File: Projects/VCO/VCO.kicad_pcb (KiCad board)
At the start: 2 copper layers, 13.2 x 38.4 mm, 33 parts, among them J1 Conn_01x02, J3 Conn_01x02, Q1 BFR193, Q2 BFR193

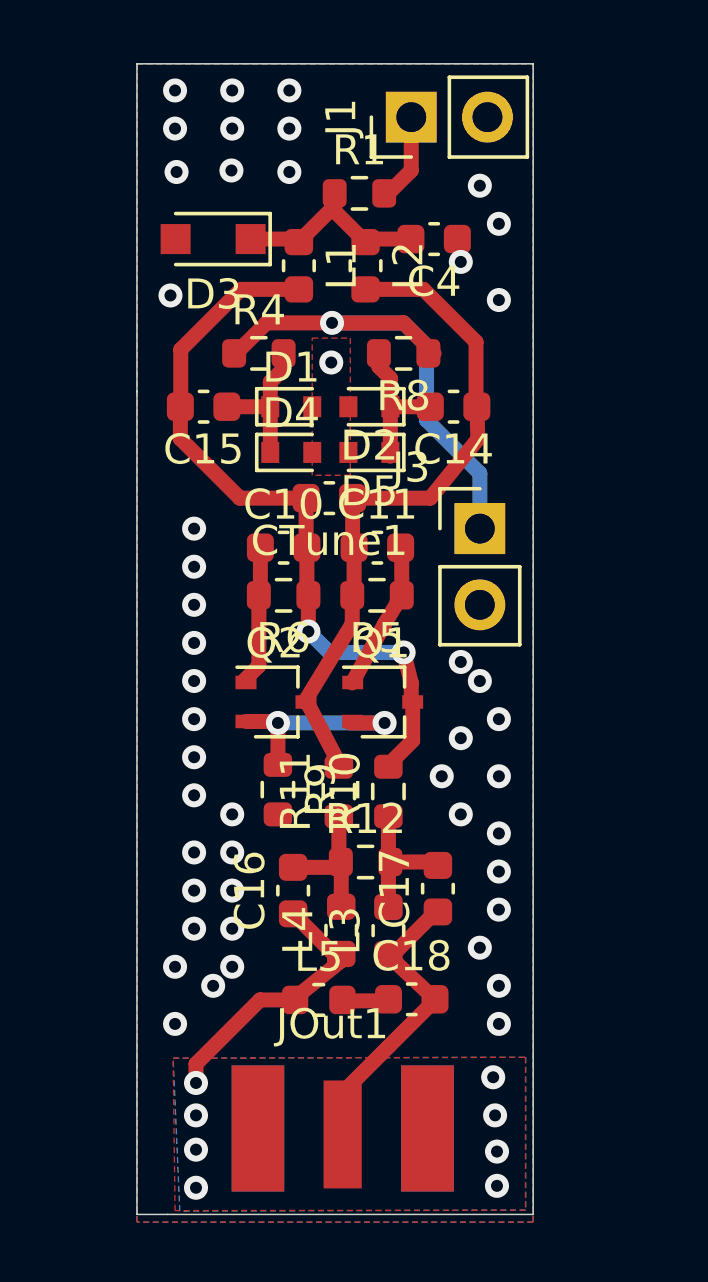
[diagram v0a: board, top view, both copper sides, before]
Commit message: last update
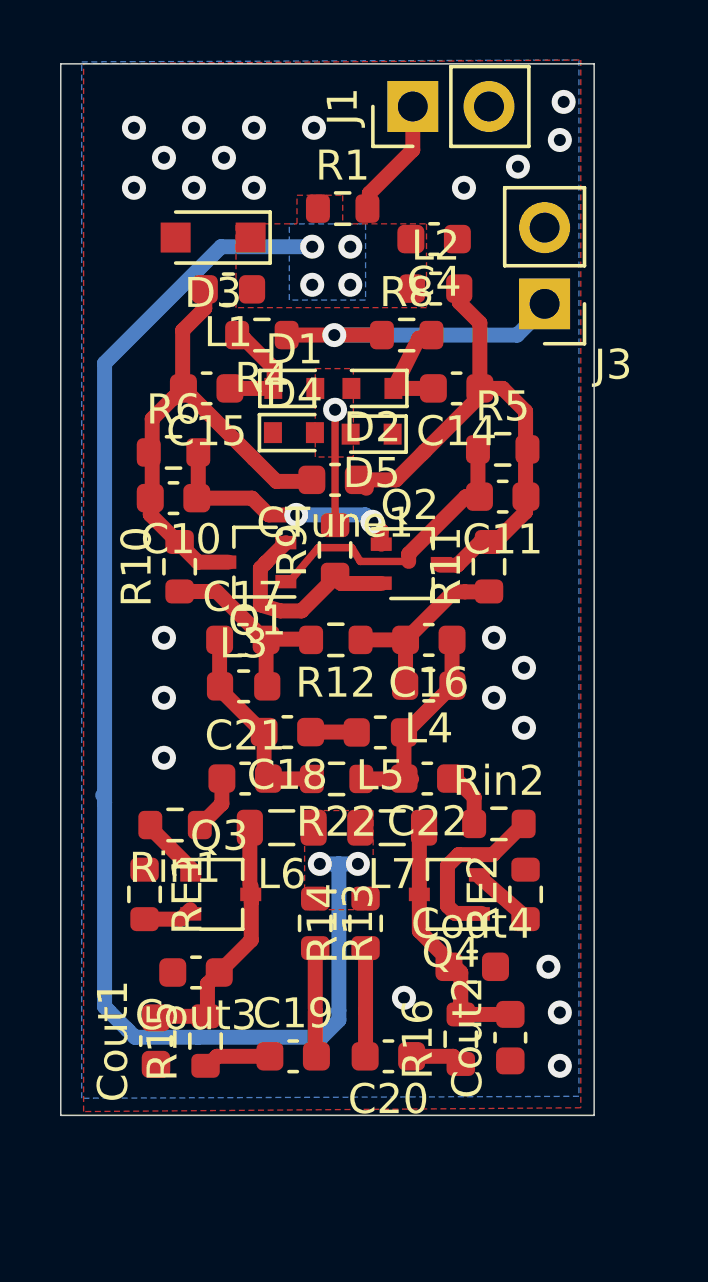
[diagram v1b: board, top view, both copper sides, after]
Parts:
- removed JOut1: SMA-J-P-H-ST-EM1, AdditionalLibs:SAMTEC_SMA-J-P-H-ST-EM1
- added C19: 1n, Capacitor_SMD:C_0603_1608Metric, F.Cu at (139.8, 63.3)
- added C20: 1n, Capacitor_SMD:C_0603_1608Metric, F.Cu at (143.0, 63.3)
- added C21: 1n, Capacitor_SMD:C_0603_1608Metric, F.Cu at (138.2, 54.1)
- added C22: 1n, Capacitor_SMD:C_0603_1608Metric, F.Cu at (144.3, 54.1)
- added Cout1: 10n, Capacitor_SMD:C_0603_1608Metric, F.Cu at (135.3, 62.8)
- added Cout2: 10n, Capacitor_SMD:C_0603_1608Metric, F.Cu at (147.1, 62.7)
- added Cout3: 22p, Capacitor_SMD:C_0603_1608Metric, F.Cu at (136.6, 60.5)
- added Cout4: 22p, Capacitor_SMD:C_0603_1608Metric, F.Cu at (145.8, 60.3)
- added L6: 1u, Inductor_SMD:L_0805_2012Metric, F.Cu at (139.4, 55.7)
- added L7: 1u, Inductor_SMD:L_0805_2012Metric, F.Cu at (143.1, 55.7)
- added Q3: BFR193, Package_TO_SOT_SMD:SOT-323_SC-70, F.Cu at (137.4, 57.9)
- added Q4: BFR193, Package_TO_SOT_SMD:SOT-323_SC-70, F.Cu at (145.0, 57.9)
- added R13: 24k, Resistor_SMD:R_0603_1608Metric, F.Cu at (140.6, 58.9)
- added R14: 24k, Resistor_SMD:R_0603_1608Metric, F.Cu at (142.2, 58.9)
- added R15: 1k, Resistor_SMD:R_0603_1608Metric, F.Cu at (136.9, 62.8)
- added R16: 1k, Resistor_SMD:R_0603_1608Metric, F.Cu at (145.4, 62.7)
- added R22: 330, Resistor_SMD:R_0603_1608Metric, F.Cu at (141.3, 54.1)
- added RE1: 10, Resistor_SMD:R_0603_1608Metric, F.Cu at (134.9, 57.9)
- added RE2: 10, Resistor_SMD:R_0603_1608Metric, F.Cu at (147.6, 57.9)
- added Rin1: 27, Resistor_SMD:R_0603_1608Metric, F.Cu at (135.9, 55.6)
- added Rin2: 27, Resistor_SMD:R_0603_1608Metric, F.Cu at (146.7, 55.6)
- R1: value 62 -> 56
- moved C17 10.5 mm to (138.2, 49.4), turned to 0 degrees
- moved R10 10.2 mm to (136.0, 47.0)
- moved C18 9.83 mm to (139.6, 52.5), turned to 180 degrees
- moved C16 9.50 mm to (144.3, 49.4), turned to 180 degrees
- moved L3 9.47 mm to (138.2, 51.0), turned to 0 degrees
- moved L5 9.15 mm to (142.7, 52.5), turned to 180 degrees
- moved R11 9.01 mm to (146.4, 47.0)
- moved L4 8.66 mm to (144.3, 51.0), turned to 180 degrees
- moved R9 8.21 mm to (141.2, 46.4), turned to 90 degrees
- moved J3 7.80 mm to (148.2, 38.2), turned to 180 degrees
- moved R12 7.47 mm to (141.2, 49.4), turned to 180 degrees
- moved Q2 6.45 mm to (143.8, 46.9)
- moved R5 6.42 mm to (146.8, 43.1), turned to 0 degrees
- moved Q1 6.29 mm to (138.6, 46.8), turned to 180 degrees
- moved R6 6.01 mm to (135.8, 43.2), turned to 0 degrees
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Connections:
- net Net-(C4-Pad2) renamed /V_Power
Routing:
- net /V_Power: track 7.15 -> 45.2 mm, vias 0 -> 6
- net Net-(Cout2-Pad2): track 0.00 -> 8.93 mm
- net Net-(Cout1-Pad2): track 0.00 -> 8.46 mm
- net /Vop: track 24.9 -> 17.6 mm, vias 2 -> 0
- net /Vtune: track 17.7 -> 10.4 mm
- net Net-(Q4-Pad1): track 0.00 -> 5.70 mm
- net Net-(C11-Pad2): track 5.01 -> 9.62 mm
- net Net-(C10-Pad1): track 4.67 -> 8.70 mm, vias 0 -> 2
- net GND: track 0.00 -> 3.85 mm, vias 47 -> 25
- net /Von: track 22.5 -> 18.8 mm
- net Net-(C20-Pad2): track 0.00 -> 3.62 mm
- net Net-(C17-Pad1): track 10.0 -> 6.88 mm
- net Net-(C19-Pad2): track 0.00 -> 3.05 mm
- net Net-(C19-Pad1): track 0.00 -> 2.30 mm
- net Net-(C17-Pad2): track 4.49 -> 6.74 mm
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- added copper zone on B.Cu, net /V_Power
- added copper zone on F.Cu, net /V_Power
- removed copper zone on B.Cu, net Net-(C16-Pad1)
- removed copper zone on F.Cu, net Net-(C16-Pad1)
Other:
- board size 13.2 x 38.4 mm -> 17.8 x 35.1 mm
